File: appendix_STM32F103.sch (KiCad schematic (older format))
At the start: 38 parts, among them J201 Micro_SD_Card_Det, J202 Conn_02x05_Odd_Even, J203 Conn_02x20_Top_Bottom, J204 Conn_ARM_JTAG_SWD_10, SW201 SW_Push, U201 STM32F103ZETx, U202 NTS0104PW-Q100J, U203 NTS0104PW-Q100J, X201 SG-210STF

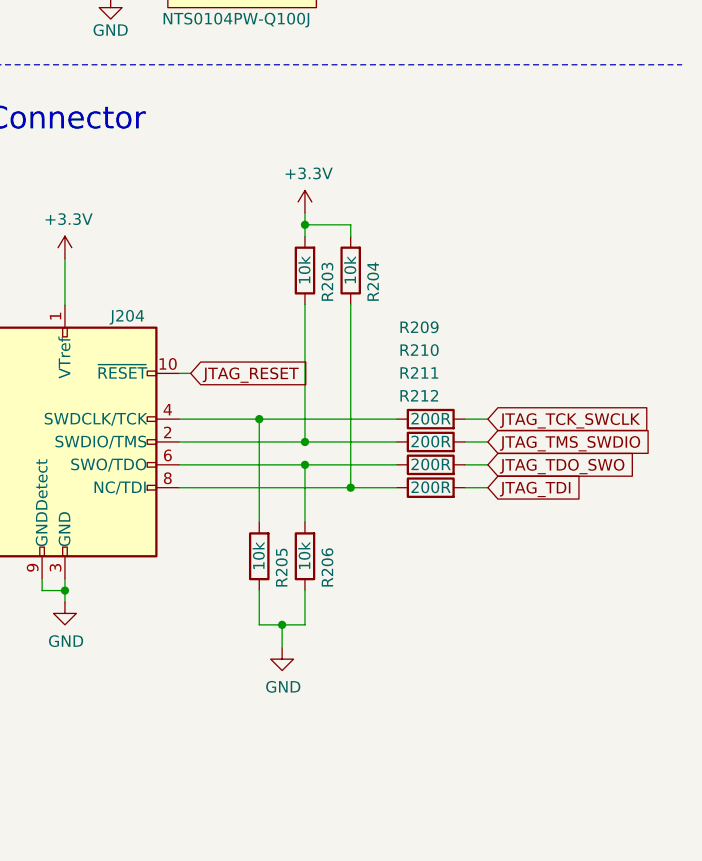
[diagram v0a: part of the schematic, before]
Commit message: added cache.lib to git
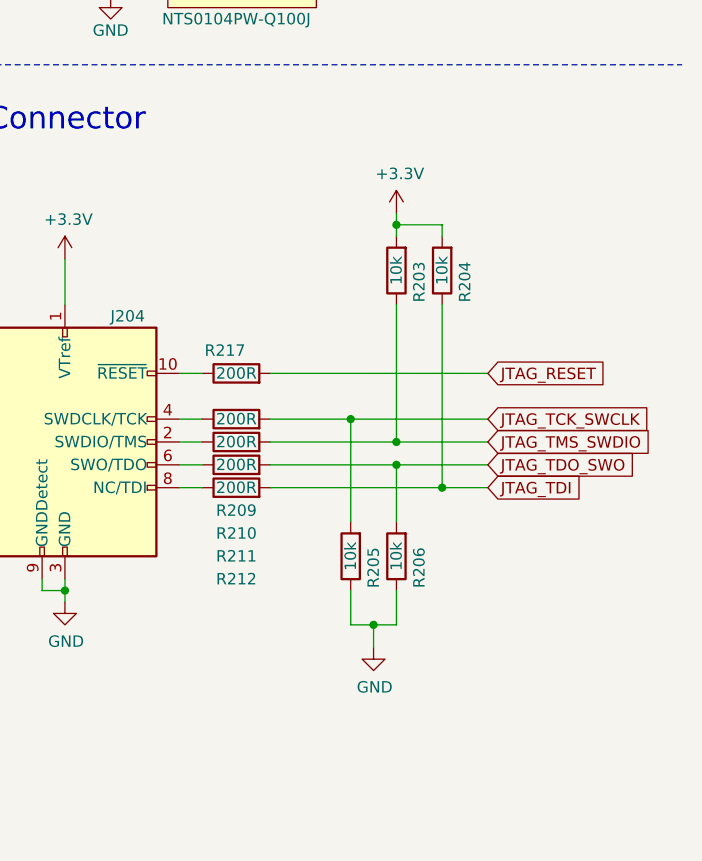
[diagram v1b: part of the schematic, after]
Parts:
- added R217: 200R, Resistors_SMD:R_0603, symbol Device:R
- J203: footprint (none) -> Connector_PinHeader_2.54mm:PinHeader_2x20_P2.54mm_Vertical
- J204: footprint (none) -> Connector_PinHeader_1.27mm:PinHeader_2x05_P1.27mm_Vertical
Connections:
- net JTAG_RESET: now also R217.2; no longer J204.10 (~RESET~)
- net JTAG_TCK_SWCLK: now also R205.2
- net JTAG_TDI: now also R204.1
- net JTAG_TDO_SWO: now also R206.2
- net JTAG_TMS_SWDIO: now also R203.1
- net at J204.2 (SWDIO/TMS), R210.1: no longer R203.1
- net at J204.8 (NC/TDI), R212.1: no longer R204.1
- net at J204.6 (SWO/TDO), R211.1: no longer R206.2
- net at J204.4 (SWDCLK/TCK), R209.1: no longer R205.2
- new net: J204.10 (~RESET~), R217.1
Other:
- moved on the sheet: R203, R204, R205, R206, R209, R210, R211, R212
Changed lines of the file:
@@
 L Device:R R203
 U 1 1 5CB89A78
-P 14400 8050
-F 0 "R203" V 14300 8100 50  0000 C CNN
-F 1 "10k" V 14400 8050 50  0000 C CNN
-F 2 "Resistors_SMD:R_0603" V 14330 8050 50  0001 C CNN
-F 3 "~" H 14400 8050 50  0001 C CNN
-	1    14400 8050
+P 14800 8050
+F 0 "R203" V 14700 8100 50  0000 C CNN
+F 1 "10k" V 14800 8050 50  0000 C CNN
+F 2 "Resistors_SMD:R_0603" V 14730 8050 50  0001 C CNN
+F 3 "~" H 14800 8050 50  0001 C CNN
+	1    14800 8050
 	-1   0    0    1
 $EndComp
@@
 L Device:R R204
 U 1 1 5CB89E62
-P 14600 8050
-F 0 "R204" V 14500 8100 50  0000 C CNN
-F 1 "10k" V 14600 8050 50  0000 C CNN
-F 2 "Resistors_SMD:R_0603" V 14530 8050 50  0001 C CNN
-F 3 "~" H 14600 8050 50  0001 C CNN
-	1    14600 8050
+P 15000 8050
+F 0 "R204" V 14900 8100 50  0000 C CNN
+F 1 "10k" V 15000 8050 50  0000 C CNN
+F 2 "Resistors_SMD:R_0603" V 14930 8050 50  0001 C CNN
+F 3 "~" H 15000 8050 50  0001 C CNN
+	1    15000 8050
 	-1   0    0    1
 $EndComp
 Wire Wire Line
-	14400 8200 14400 8800
+	14800 8200 14800 8800
 Wire Wire Line
-	14600 8200 14600 9000
+	15000 8200 15000 9000
 Wire Wire Line
-	14600 9000 14800 9000
+	15000 9000 15200 9000
 Wire Wire Line
-	14400 8800 14800 8800
+	14800 8800 15200 8800
 $Comp
 L Device:R R206
 U 1 1 5CBAA3AC
-P 14400 9300
-F 0 "R206" V 14300 9350 50  0000 C CNN
-F 1 "10k" V 14400 9300 50  0000 C CNN
-F 2 "Resistors_SMD:R_0603" V 14330 9300 50  0001 C CNN
-F 3 "~" H 14400 9300 50  0001 C CNN
-	1    14400 9300
+P 14800 9300
+F 0 "R206" V 14700 9350 50  0000 C CNN
+F 1 "10k" V 14800 9300 50  0000 C CNN
+F 2 "Resistors_SMD:R_0603" V 14730 9300 50  0001 C CNN
+F 3 "~" H 14800 9300 50  0001 C CNN
+	1    14800 9300
 	-1   0    0    1
 $EndComp
 Wire Wire Line
-	14400 9150 14400 8900
+	14800 9150 14800 8900
 Wire Wire Line
-	14400 8900 14800 8900
+	14800 8900 15200 8900
 $Comp
 L Device:R R205
 U 1 1 5CBAEA23
-P 14200 9300
-F 0 "R205" V 14100 9350 50  0000 C CNN
-F 1 "10k" V 14200 9300 50  0000 C CNN
-F 2 "Resistors_SMD:R_0603" V 14130 9300 50  0001 C CNN
-F 3 "~" H 14200 9300 50  0001 C CNN
-	1    14200 9300
+P 14600 9300
+F 0 "R205" V 14500 9350 50  0000 C CNN
+F 1 "10k" V 14600 9300 50  0000 C CNN
+F 2 "Resistors_SMD:R_0603" V 14530 9300 50  0001 C CNN
+F 3 "~" H 14600 9300 50  0001 C CNN
+	1    14600 9300
 	-1   0    0    1
 $EndComp
 Wire Wire Line
-	14200 9150 14200 8700
+	14600 9150 14600 8700
 Wire Wire Line
-	14200 8700 14800 8700
+	14600 8700 15200 8700
 $Comp
 L power:GND #PWR0119
 U 1 1 5CBB26E4
-P 14300 9700
-F 0 "#PWR0119" H 14300 9450 50  0001 C CNN
-F 1 "GND" H 14305 9527 50  0000 C CNN
-F 2 "" H 14300 9700 50  0001 C CNN
-F 3 "" H 14300 9700 50  0001 C CNN
-	1    14300 9700
+P 14700 9700
+F 0 "#PWR0119" H 14700 9450 50  0001 C CNN
+F 1 "GND" H 14705 9527 50  0000 C CNN
+F 2 "" H 14700 9700 50  0001 C CNN
+F 3 "" H 14700 9700 50  0001 C CNN
+	1    14700 9700
 	1    0    0    -1
 $EndComp
 Wire Wire Line
-	14200 9450 14200 9600
+	14600 9450 14600 9600
 Wire Wire Line
-	14200 9600 14300 9600
+	14600 9600 14700 9600
 Wire Wire Line
-	14400 9600 14400 9450
+	14800 9600 14800 9450
 Wire Wire Line
-	14300 9600 14300 9700
-Connection ~ 14300 9600
+	14700 9600 14700 9700
+Connection ~ 14700 9600
 Wire Wire Line
-	14300 9600 14400 9600
+	14700 9600 14800 9600
 $Comp
 L power:+3.3V #PWR0120
 U 1 1 5CBBABAF
-P 14400 7800
-F 0 "#PWR0120" H 14400 7650 50  0001 C CNN
-F 1 "+3.3V" H 14415 7973 50  0000 C CNN
-F 2 "" H 14400 7800 50  0001 C CNN
-F 3 "" H 14400 7800 50  0001 C CNN
-	1    14400 7800
+P 14800 7800
+F 0 "#PWR0120" H 14800 7650 50  0001 C CNN
+F 1 "+3.3V" H 14815 7973 50  0000 C CNN
+F 2 "" H 14800 7800 50  0001 C CNN
+F 3 "" H 14800 7800 50  0001 C CNN
+	1    14800 7800
 	1    0    0    -1
 $EndComp
 Wire Wire Line
-	14600 7900 14600 7850
+	15000 7900 15000 7850
 Wire Wire Line
-	14600 7850 14400 7850
+	15000 7850 14800 7850
 Wire Wire Line
-	14400 7900 14400 7850
-Connection ~ 14400 7850
+	14800 7900 14800 7850
+Connection ~ 14800 7850
 Wire Wire Line
-	14400 7850 14400 7800
+	14800 7850 14800 7800
 $Comp
 L power:+3.3VA #PWR0123
@@
 F 0 "J204" H 13700 9350 50  0000 R CNN
 F 1 "Conn_ARM_JTAG_SWD_10" V 12900 9250 50  0000 R CNN
-F 2 "" H 13350 8800 50  0001 C CNN
+F 2 "Connector_PinHeader_1.27mm:PinHeader_2x05_P1.27mm_Vertical" H 13350 8800 50  0001 C CNN
 F 3 "http://infocenter.arm.com/help/topic/com.arm.doc.ddi0314h/DDI0314H_coresight_components_trm.pdf" V 13000 7550 50  0001 C CNN
 	1    13350 8800
@@
 Wire Wire Line
 	13350 9450 13350 9400
-Wire Wire Line
-	13850 8500 13900 8500
-Text GLabel 13900 8500 2    50   Input ~ 0
+Text GLabel 15200 8500 2    50   Input ~ 0
 JTAG_RESET
 $Comp
@@
 Wire Wire Line
 	14850 5000 14650 5000
-Wire Wire Line
-	13850 8700 14200 8700
-Connection ~ 14200 8700
-Wire Wire Line
-	14400 8800 13850 8800
-Connection ~ 14400 8800
-Wire Wire Line
-	13850 8900 14400 8900
-Connection ~ 14400 8900
-Wire Wire Line
-	14600 9000 13850 9000
-Connection ~ 14600 9000
 $Comp
 L Device:R R212
 U 1 1 5CD04150
-P 14950 9000
-F 0 "R212" V 15350 9050 50  0000 C CNN
-F 1 "200R" V 14950 9000 50  0000 C CNN
-F 2 "Resistors_SMD:R_0603" V 14880 9000 50  0001 C CNN
-F 3 "~" H 14950 9000 50  0001 C CNN
-	1    14950 9000
+P 14100 9000
+F 0 "R212" V 13700 9000 50  0000 C CNN
+F 1 "200R" V 14100 9000 50  0000 C CNN
+F 2 "Resistors_SMD:R_0603" V 14030 9000 50  0001 C CNN
+F 3 "~" H 14100 9000 50  0001 C CNN
+	1    14100 9000
 	0    -1   -1   0
 $EndComp
@@
 L Device:R R211
 U 1 1 5CD05002
-P 14950 8900
-F 0 "R211" V 15350 8950 50  0000 C CNN
-F 1 "200R" V 14950 8900 50  0000 C CNN
-F 2 "Resistors_SMD:R_0603" V 14880 8900 50  0001 C CNN
-F 3 "~" H 14950 8900 50  0001 C CNN
-	1    14950 8900
+P 14100 8900
+F 0 "R211" V 13700 8900 50  0000 C CNN
+F 1 "200R" V 14100 8900 50  0000 C CNN
+F 2 "Resistors_SMD:R_0603" V 14030 8900 50  0001 C CNN
+F 3 "~" H 14100 8900 50  0001 C CNN
+	1    14100 8900
 	0    -1   -1   0
 $EndComp
@@
 L Device:R R210
 U 1 1 5CD0523F
-P 14950 8800
-F 0 "R210" V 15350 8850 50  0000 C CNN
-F 1 "200R" V 14950 8800 50  0000 C CNN
-F 2 "Resistors_SMD:R_0603" V 14880 8800 50  0001 C CNN
-F 3 "~" H 14950 8800 50  0001 C CNN
-	1    14950 8800
+P 14100 8800
+F 0 "R210" V 13700 8800 50  0000 C CNN
+F 1 "200R" V 14100 8800 50  0000 C CNN
+F 2 "Resistors_SMD:R_0603" V 14030 8800 50  0001 C CNN
+F 3 "~" H 14100 8800 50  0001 C CNN
+	1    14100 8800
 	0    -1   -1   0
 $EndComp
@@
 L Device:R R209
 U 1 1 5CD053EB
-P 14950 8700
-F 0 "R209" V 15350 8750 50  0000 C CNN
-F 1 "200R" V 14950 8700 50  0000 C CNN
-F 2 "Resistors_SMD:R_0603" V 14880 8700 50  0001 C CNN
-F 3 "~" H 14950 8700 50  0001 C CNN
-	1    14950 8700
+P 14100 8700
+F 0 "R209" V 13700 8700 50  0000 C CNN
+F 1 "200R" V 14100 8700 50  0000 C CNN
+F 2 "Resistors_SMD:R_0603" V 14030 8700 50  0001 C CNN
+F 3 "~" H 14100 8700 50  0001 C CNN
+	1    14100 8700
 	0    -1   -1   0
 $EndComp
 Wire Wire Line
-	15100 8700 15200 8700
-Wire Wire Line
-	15100 8800 15200 8800
-Wire Wire Line
-	15100 8900 15200 8900
-Wire Wire Line
-	15100 9000 15200 9000
-Wire Wire Line
 	14550 3950 14300 3950
 Wire Wire Line
@@
 F 0 "J203" H 6850 10900 50  0000 C CNN
 F 1 "Conn_02x20_Top_Bottom" H 6850 11100 50  0000 C CNN
-F 2 "" H 6800 9850 50  0001 C CNN
+F 2 "Connector_PinHeader_2.54mm:PinHeader_2x20_P2.54mm_Vertical" H 6800 9850 50  0001 C CNN
 F 3 "~" H 6800 9850 50  0001 C CNN
 	1    6800 9850
@@
 	1    0    0    -1
 $EndComp
+Wire Wire Line
+	13850 8700 13950 8700
+Wire Wire Line
+	13850 8800 13950 8800
+Wire Wire Line
+	13950 8900 13850 8900
+Wire Wire Line
+	13850 9000 13950 9000
+Wire Wire Line
+	14250 8700 14600 8700
+Connection ~ 14600 8700
+Wire Wire Line
+	14800 8800 14250 8800
+Connection ~ 14800 8800
+Wire Wire Line
+	14250 8900 14800 8900
+Connection ~ 14800 8900
+Wire Wire Line
+	15000 9000 14250 9000
+Connection ~ 15000 9000
+$Comp
+L Device:R R217
+U 1 1 5CDCD7F7
+P 14100 8500
+F 0 "R217" V 14200 8550 50  0000 C CNN
+F 1 "200R" V 14100 8500 50  0000 C CNN
+F 2 "Resistors_SMD:R_0603" V 14030 8500 50  0001 C CNN
+F 3 "~" H 14100 8500 50  0001 C CNN
+	1    14100 8500
+	0    -1   -1   0
+$EndComp
+Wire Wire Line
+	13850 8500 13950 8500
+Wire Wire Line
+	14250 8500 15200 8500
 $EndSCHEMATC
